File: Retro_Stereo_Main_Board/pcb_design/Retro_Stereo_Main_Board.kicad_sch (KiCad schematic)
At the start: 16 parts, among them J1 BM23FR0.6-30DS-0.35V895, J2 USB_C_Receptacle, J3 1734366-1, J4 SD_Card_Receptacle, J5 TC2030, J6 Conn_01x04, J7 Conn_01x06, J8 Conn_01x06, SW1 RotaryEncoder_Switch_MP, SW9 SW_Push

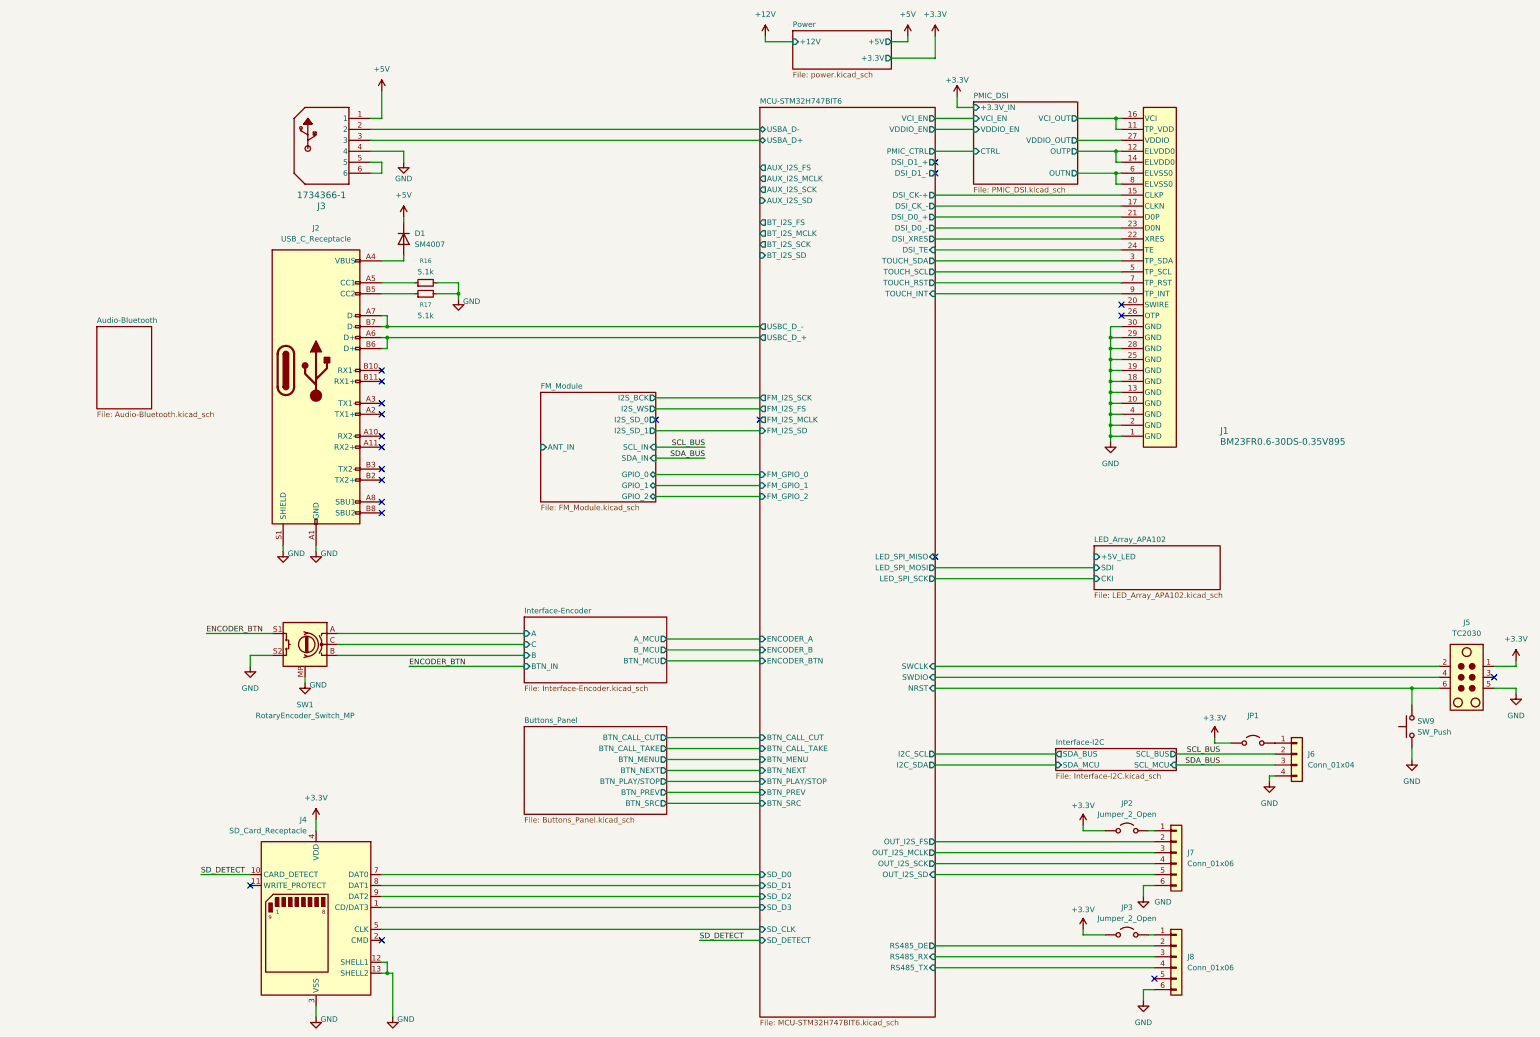
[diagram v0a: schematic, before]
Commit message: Complete BT module sheet
Signed-off-by: Francisco <fran.testa07Qgmail.com>
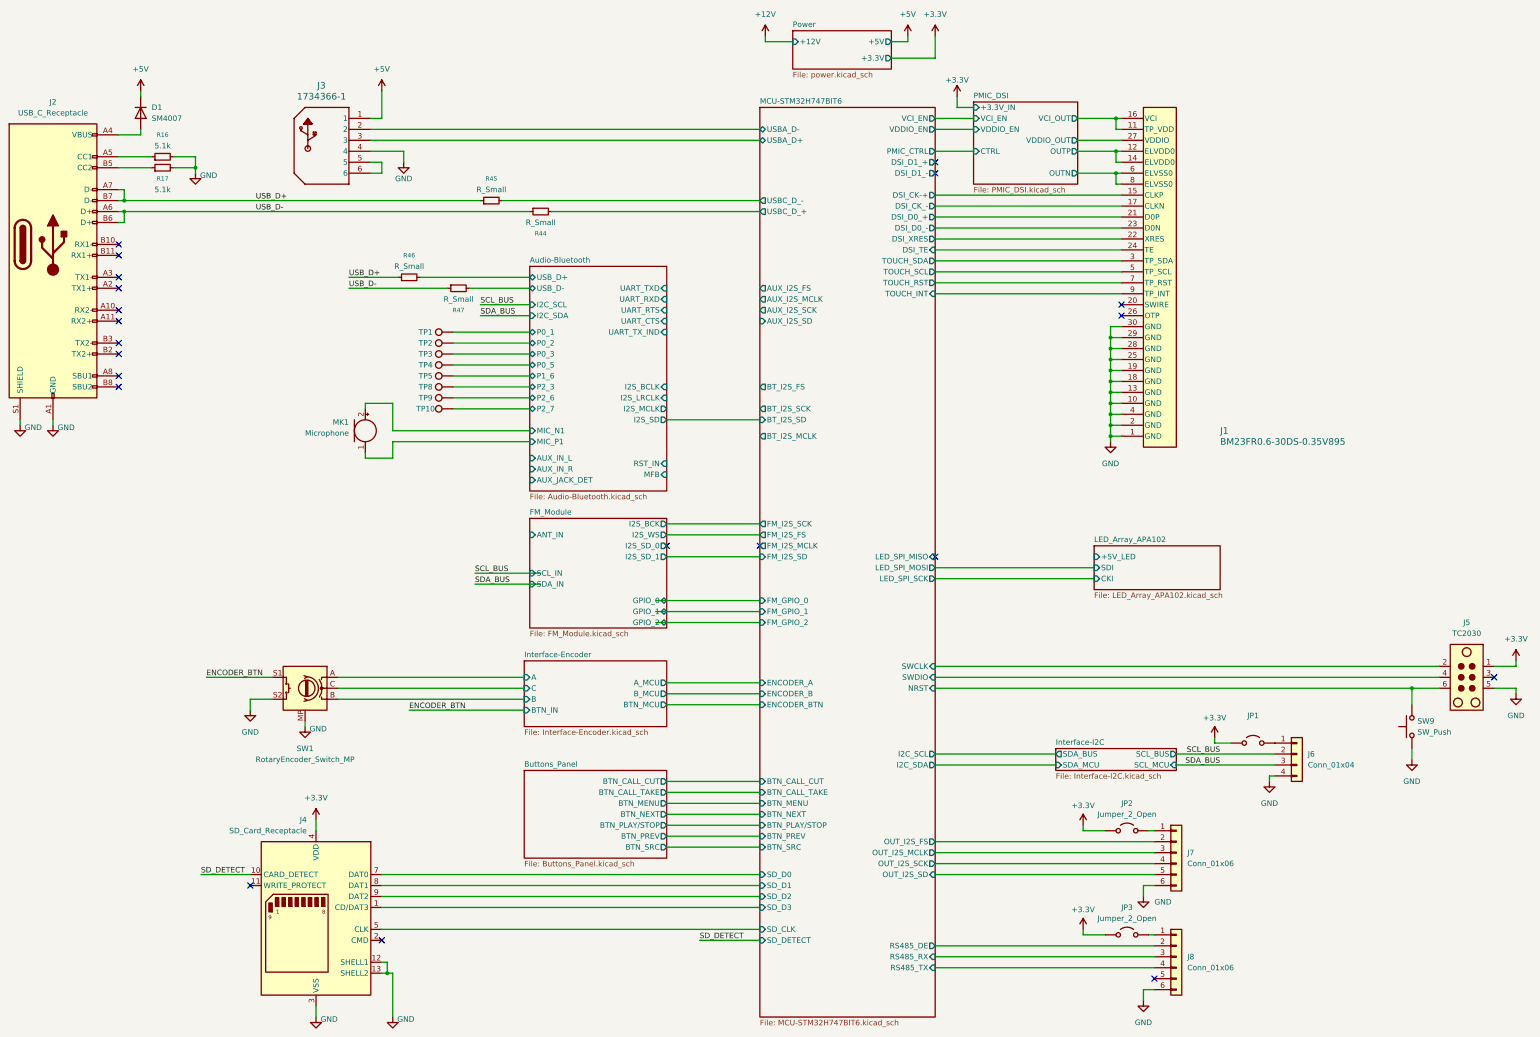
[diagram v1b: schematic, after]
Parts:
- added MK1: Microphone, symbol Device:Microphone
- added R44, R45, R46, R47: R_Small, symbol Device:R_Small
- added TP1, TP10, TP2, TP3, TP4, TP5, TP8, TP9: TestPoint, symbol Connector:TestPoint
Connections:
- net MCU-STM32H747BIT6/USBC_D_+: now also R44.2; no longer J2.A6 (D+), J2.B6 (D+)
- net MCU-STM32H747BIT6/USBC_D_-: now also R45.2; no longer J2.A7 (D-), J2.B7 (D-)
- new net Audio-Bluetooth/MIC_N1: MK1.2 (+)
- new net Audio-Bluetooth/MIC_P1: MK1.1 (-)
- new net Audio-Bluetooth/P0_1: TP1.1
- new net Audio-Bluetooth/P0_2: TP2.1
- new net Audio-Bluetooth/P0_3: TP3.1
- new net Audio-Bluetooth/P0_5: TP4.1
- new net Audio-Bluetooth/P1_6: TP5.1
- new net Audio-Bluetooth/P2_3: TP8.1
- new net Audio-Bluetooth/P2_6: TP9.1
- new net Audio-Bluetooth/P2_7: TP10.1
- new net Audio-Bluetooth/USB_D+: R46.2
- new net Audio-Bluetooth/USB_D-: R47.2
- new net USB_D+: J2.A7 (D-), J2.B7 (D-), R45.1, R46.1
- new net USB_D-: J2.A6 (D+), J2.B6 (D+), R44.1, R47.1
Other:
- sheet Audio-Bluetooth ports: added AUX_IN_L, AUX_IN_R, AUX_JACK_DET, I2C_SCL, I2C_SDA, I2S_BCLK, I2S_LRCLK, I2S_MCLK, I2S_SD, MFB, MIC_N1, MIC_P1, P0_1, P0_2, P0_3, P0_5, P1_6, P2_3, P2_6, P2_7, RST_IN, UART_CTS, UART_RTS, UART_RXD, UART_TXD, UART_TX_IND, USB_D+, USB_D-; removed none
- moved on the sheet: D1, J2, R16, R17, SW1
